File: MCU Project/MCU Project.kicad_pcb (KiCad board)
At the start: 2 copper layers, 75.5 x 38.5 mm, 15 parts, among them J1 CONBNC001, J2 CONBNC001, U1 LSHD-5601, U3 1825966-1, U4 1825966-1

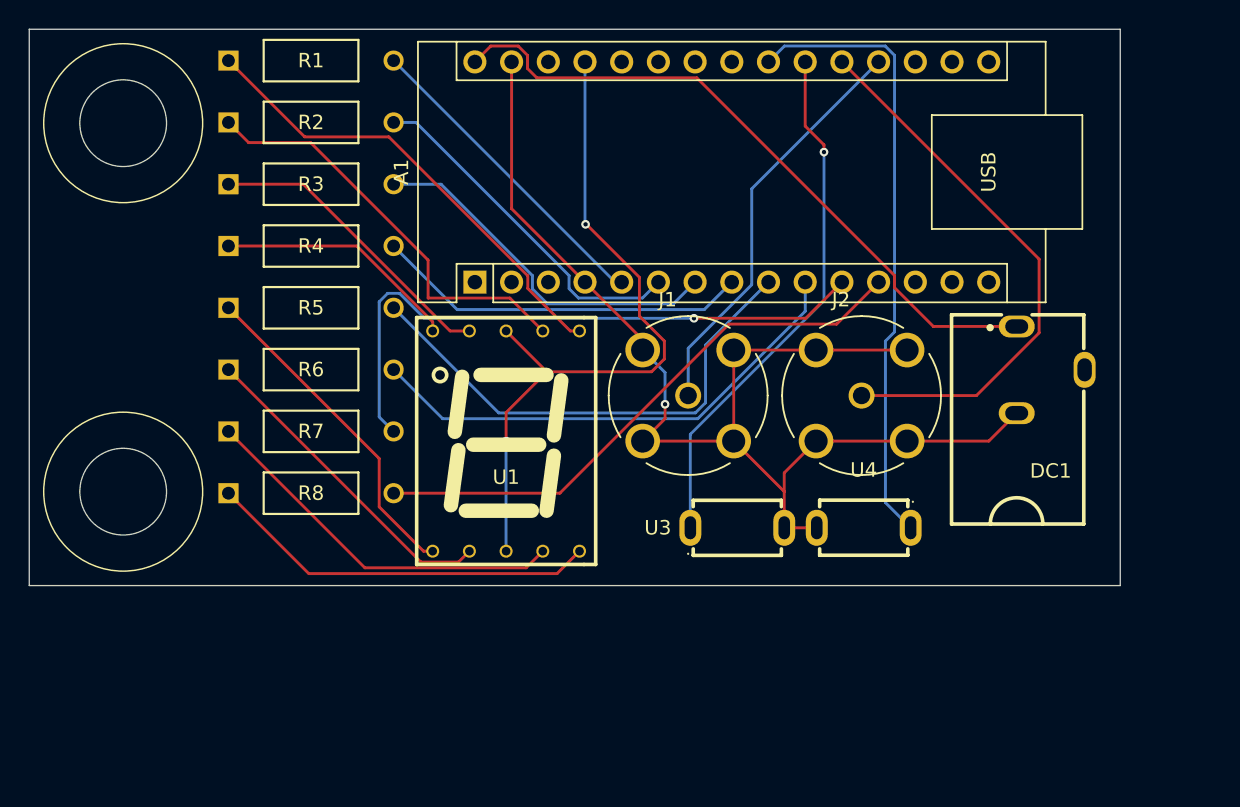
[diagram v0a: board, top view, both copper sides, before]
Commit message: Do something
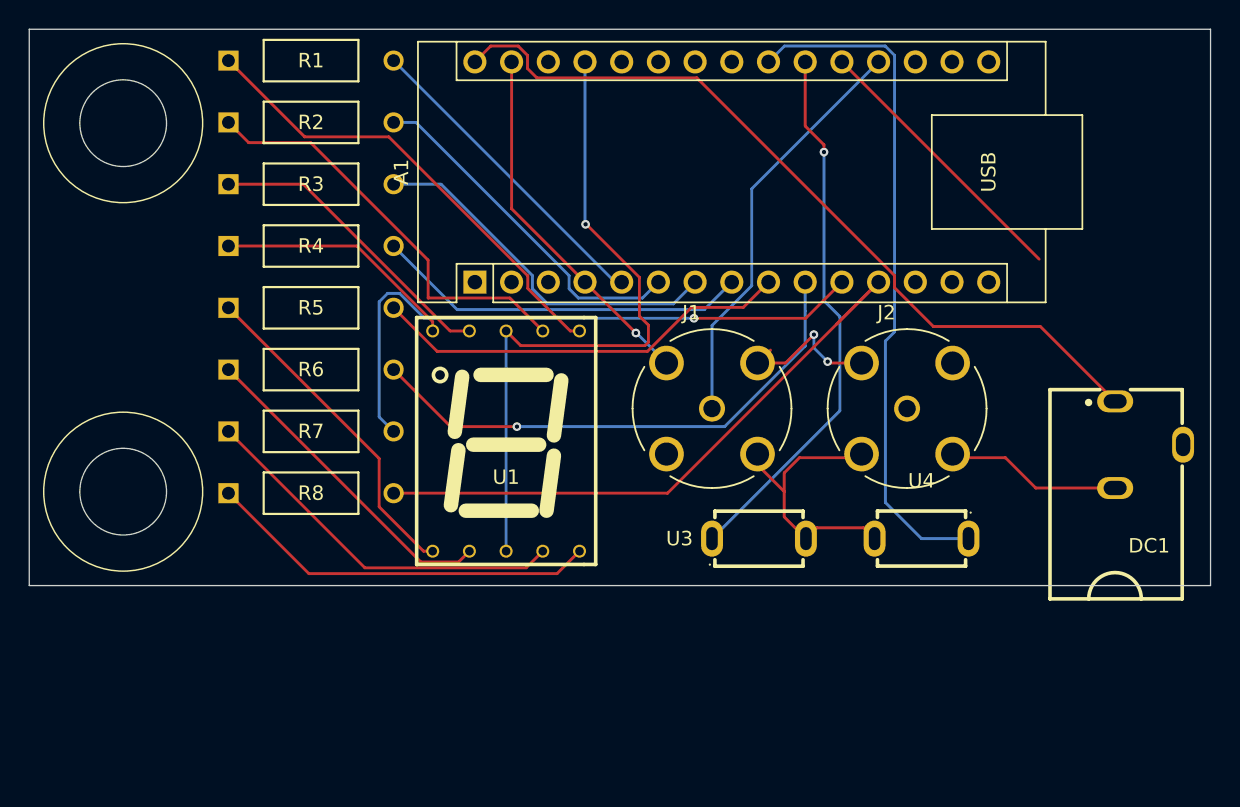
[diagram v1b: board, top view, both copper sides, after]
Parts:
- moved DC1 8.56 mm to (176.5, 104.8)
- moved U4 4.07 mm to (160.8, 111.2)
- moved J2 3.28 mm to (159.8, 102.2)
- moved J1 1.88 mm to (146.2, 102.2)
- moved U3 1.68 mm to (149.5, 111.2)
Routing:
- net Net-(A1-A1): track 38.5 -> 19.3 mm
- net GND: track 84.7 -> 68.0 mm, vias 1 -> 3
- net Net-(A1-VIN): track 47.0 -> 56.0 mm
- net Net-(A1-D6): track 35.0 -> 29.2 mm
- net Net-(A1-A3): track 43.1 -> 47.4 mm
- net Net-(A1-D9): track 39.6 -> 43.7 mm
- net +5V: track 48.9 -> 46.9 mm, vias 2 -> 1
- net Net-(A1-D7): track 35.0 -> 36.9 mm, vias 0 -> 1
- net Net-(A1-A2): track 36.6 -> 37.6 mm
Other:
- board size 75.5 x 38.5 mm -> 81.8 x 38.5 mm

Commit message: Do something
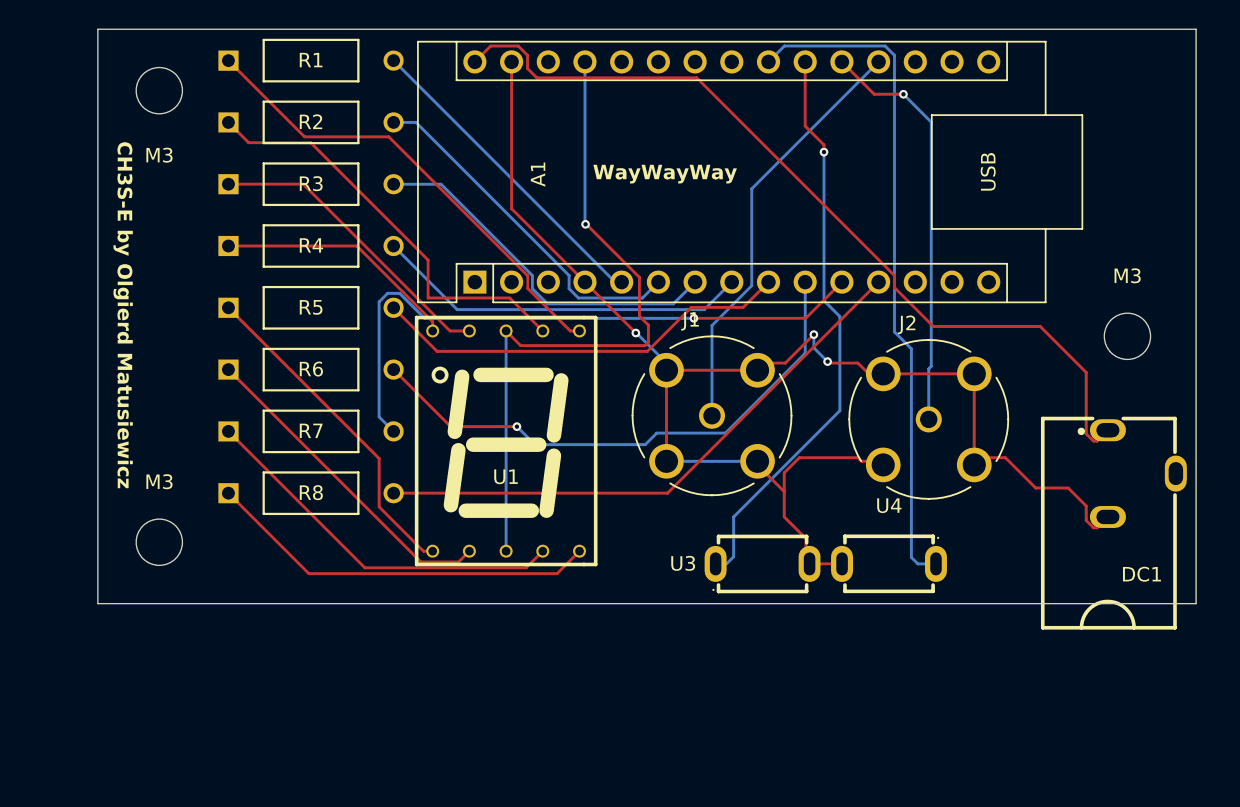
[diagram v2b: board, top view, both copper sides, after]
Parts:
- added M3: MountingHole_3.2mm_M3, MountingHole:MountingHole_3.2mm_M3, F.Cu at (175.0, 97.2)
- added M3: MountingHole_3.2mm_M3, MountingHole:MountingHole_3.2mm_M3, F.Cu at (108.0, 111.5)
- added M3: MountingHole_3.2mm_M3, MountingHole:MountingHole_3.2mm_M3, F.Cu at (108.0, 80.2)
- moved U4 2.85 mm to (158.5, 113.0)
- moved DC1 2.06 mm to (176.0, 106.8)
- moved U3 1.77 mm to (149.8, 113.0)
- moved J2 1.68 mm to (161.2, 103.0)
- moved J1 0.50 mm to (146.2, 102.8)
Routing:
- net GND: track 68.0 -> 101.3 mm
- net Net-(A1-A1): track 19.3 -> 28.6 mm, vias 0 -> 1
- net Net-(A1-D9): track 43.7 -> 39.6 mm
- net Net-(A1-VIN): track 56.0 -> 59.4 mm
- net Net-(A1-A2): track 37.6 -> 39.7 mm
- net Net-(A1-D7): track 36.9 -> 38.2 mm
- net Net-(A1-A3): track 47.4 -> 46.6 mm
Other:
- board size 81.8 x 38.5 mm -> 76 x 39.8 mm
- board text added: "CH3S-E by Olgierd Matusiewicz"
- board text added: "WayWayWay"

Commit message: Do something
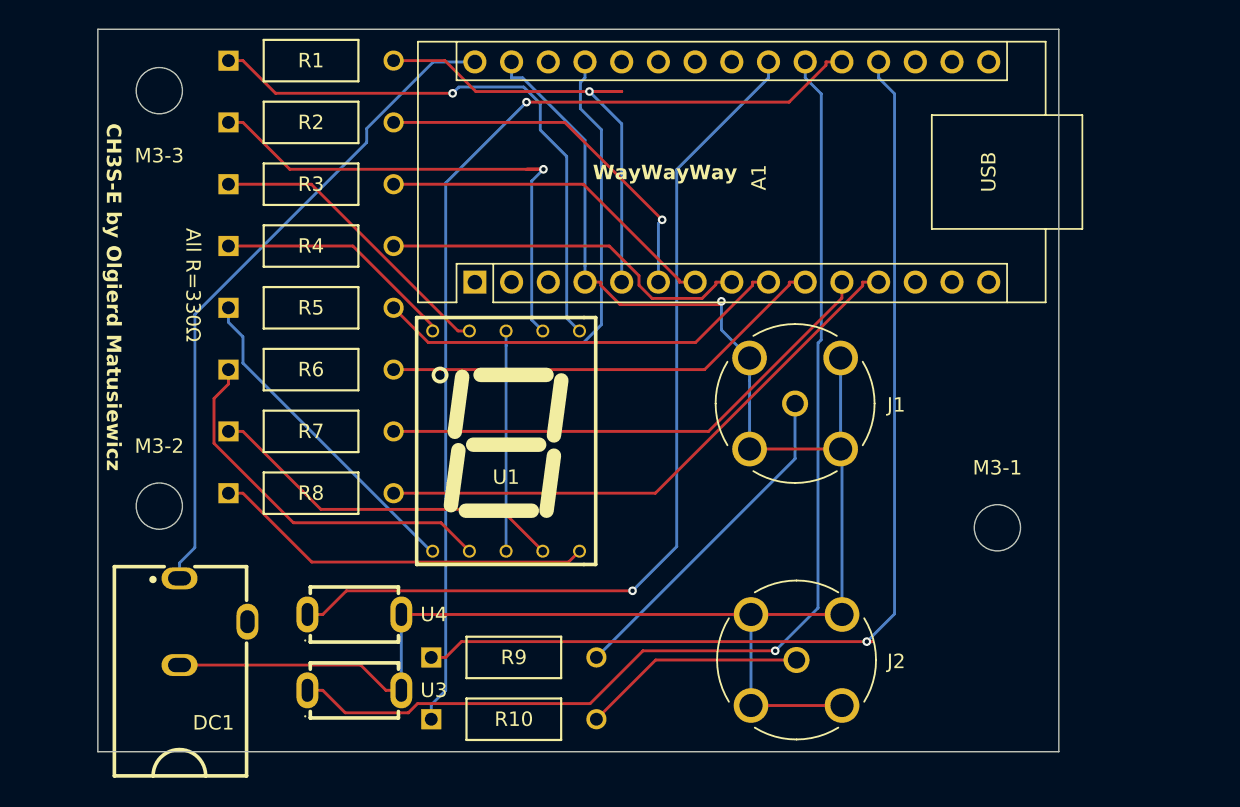
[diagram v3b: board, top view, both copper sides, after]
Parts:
- added R10: CF14JT330R, Snapeda:STA_CF14_STP, F.Cu at (126.8, 123.8)
- added R9: CF14JT330R, Snapeda:STA_CF14_STP, F.Cu at (126.8, 119.5)
- A1: footprint Microprocessors:Arduino_Nano_With_3DModel -> Module:Arduino_Nano
- moved DC1 65.1 mm to (111.8, 117.0)
- moved U4 37.2 mm to (121.5, 116.5), turned to 180 degrees
- moved U3 29.6 mm to (121.5, 121.8)
- moved J2 19.0 mm to (152.1, 119.7)
- moved M3-1 16.0 mm to (166.0, 110.5)
- moved J1 5.81 mm to (152.0, 101.9)
- moved M3-2 2.50 mm to (108.0, 109.0)
- renumbered M3 to M3-1, M3 to M3-2, M3 to M3-3
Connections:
- J1 pad 1: Net-(A1-A0) -> Net-(J1-Pad1)
- J2 pad 1: Net-(A1-A1) -> Net-(J2-Pad1)
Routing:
- net Net-(A1-A0): track 29.3 -> 73.5 mm, vias 0 -> 1
- net Net-(A1-A1): track 28.6 -> 68.6 mm
- net Net-(A1-A2): track 39.7 -> 77.3 mm
- net GND: track 101.3 -> 128.9 mm, vias 3 -> 1
- net Net-(J1-Pad1): track 0.00 -> 23.3 mm
- net Net-(A1-A3): track 46.6 -> 63.7 mm, vias 0 -> 1
- net Net-(J2-Pad1): track 0.00 -> 15.5 mm
- net Net-(A1-D2): track 22.1 -> 37.5 mm, vias 0 -> 1
- net Net-(A1-VIN): track 59.4 -> 45.9 mm
- net Net-(U1-D): track 29.3 -> 39.6 mm, vias 0 -> 1
- net Net-(U1-E): track 32.6 -> 40.0 mm, vias 0 -> 1
- net Net-(A1-D8): track 43.4 -> 35.9 mm, vias 1 -> 0
- net Net-(A1-D7): track 38.2 -> 31.1 mm, vias 1 -> 0
- net +5V: track 46.9 -> 41.3 mm, vias 1 -> 0
- net Net-(U1-A): track 22.5 -> 26.3 mm
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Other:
- board size 76 x 39.8 mm -> 66.5 x 50 mm
- board text added: "All R=330Ω"
